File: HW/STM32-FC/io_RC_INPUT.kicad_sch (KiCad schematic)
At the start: 9 parts, among them J6 PWM_Conn_3x14, J7 ZH 1.5mm 3P, J8 ZH 1.5mm 4P, Q2 S9013

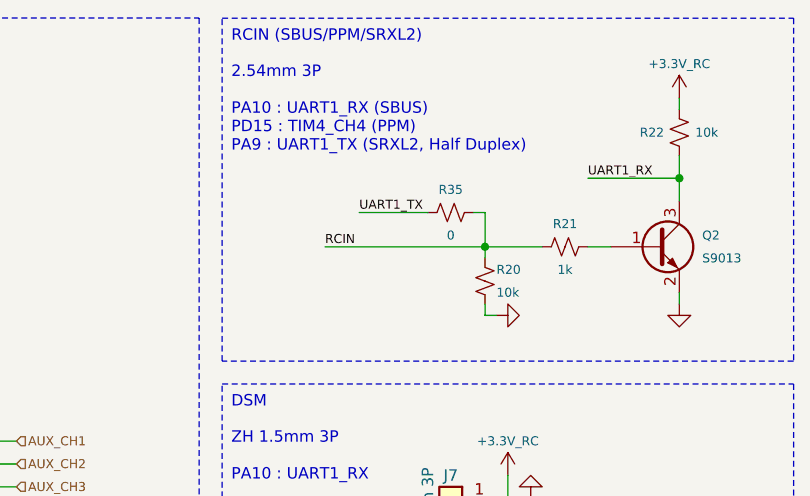
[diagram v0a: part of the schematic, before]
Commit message: 2025.02.05 PCB routing done
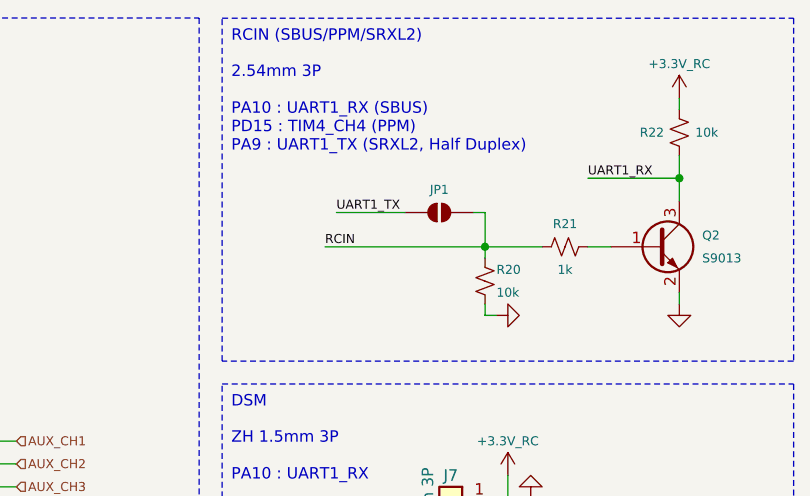
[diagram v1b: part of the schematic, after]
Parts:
- removed R35: 0, Resistor_SMD:R_0402_1005Metric, symbol Device:R_Small_US
- added JP1: SolderJumper_2_Open, Jumper:SolderJumper-2_P1.3mm_Open_TrianglePad1.0x1.5mm, symbol Jumper:SolderJumper_2_Open
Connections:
- net PPM_IN: now also JP1.2 (B)
- net UART1_TX: now also JP1.1 (A)
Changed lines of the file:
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@@
 	(title_block
 		(title "RC_INPUT")
-		(date "2025-01-03")
+		(date "2025-02-05")
 		(rev "A")
 		(company "NARAE")
@@
 	(wire
 		(pts
-			(xy 104.14 34.29) (xy 111.76 34.29)
+			(xy 101.6 34.29) (xy 109.22 34.29)
 		)
 		(stroke
@@
 	)
 	(label "UART1_TX"
-		(at 104.14 34.29 0)
+		(at 101.6 34.29 0)
 		(effects
 			(font
@@
 				(path "/8d4cc317-3933-4aa6-844b-8c5c635e89c7/77caf73d-b7f5-48a6-9de3-ef3df69ee7d9"
 					(reference "#PWR076")
-					(unit 1)
-				)
-			)
-		)
-	)
-	(symbol
-		(lib_id "Device:R_Small_US")
-		(at 114.3 34.29 90)
-		(unit 1)
-		(exclude_from_sim no)
-		(in_bom yes)
-		(on_board yes)
-		(dnp no)
-		(property "Reference" "R35"
-			(at 114.3 31.75 90)
-			(effects
-				(font
-					(size 1 1)
-				)
-			)
-		)
-		(property "Value" "0"
-			(at 114.3 36.83 90)
-			(effects
-				(font
-					(size 1 1)
-				)
-			)
-		)
-		(property "Footprint" "Resistor_SMD:R_0402_1005Metric"
-			(at 114.3 34.29 0)
-			(effects
-				(font
-					(size 1.27 1.27)
-				)
-				(hide yes)
-			)
-		)
-		(property "Datasheet" "~"
-			(at 114.3 34.29 0)
-			(effects
-				(font
-					(size 1.27 1.27)
-				)
-				(hide yes)
-			)
-		)
-		(property "Description" "Resistor, small US symbol"
-			(at 114.3 34.29 0)
-			(effects
-				(font
-					(size 1.27 1.27)
-				)
-				(hide yes)
-			)
-		)
-		(property "Availability" ""
-			(at 114.3 34.29 0)
-			(effects
-				(font
-					(size 1.27 1.27)
-				)
-				(hide yes)
-			)
-		)
-		(property "Check_prices" ""
-			(at 114.3 34.29 0)
-			(effects
-				(font
-					(size 1.27 1.27)
-				)
-				(hide yes)
-			)
-		)
-		(property "Description_1" ""
-			(at 114.3 34.29 0)
-			(effects
-				(font
-					(size 1.27 1.27)
-				)
-				(hide yes)
-			)
-		)
-		(property "MF" ""
-			(at 114.3 34.29 0)
-			(effects
-				(font
-					(size 1.27 1.27)
-				)
-				(hide yes)
-			)
-		)
-		(property "MP" ""
-			(at 114.3 34.29 0)
-			(effects
-				(font
-					(size 1.27 1.27)
-				)
-				(hide yes)
-			)
-		)
-		(property "Package" ""
-			(at 114.3 34.29 0)
-			(effects
-				(font
-					(size 1.27 1.27)
-				)
-				(hide yes)
-			)
-		)
-		(property "Price" ""
-			(at 114.3 34.29 0)
-			(effects
-				(font
-					(size 1.27 1.27)
-				)
-				(hide yes)
-			)
-		)
-		(property "SnapEDA_Link" ""
-			(at 114.3 34.29 0)
-			(effects
-				(font
-					(size 1.27 1.27)
-				)
-				(hide yes)
-			)
-		)
-		(property "Sim.Device" ""
-			(at 114.3 34.29 0)
-			(effects
-				(font
-					(size 1.27 1.27)
-				)
-				(hide yes)
-			)
-		)
-		(property "Sim.Pins" ""
-			(at 114.3 34.29 0)
-			(effects
-				(font
-					(size 1.27 1.27)
-				)
-				(hide yes)
-			)
-		)
-		(pin "1"
-		)
-		(pin "2"
-		)
-		(instances
-			(project "STM32-FC"
-				(path "/8d4cc317-3933-4aa6-844b-8c5c635e89c7/77caf73d-b7f5-48a6-9de3-ef3df69ee7d9"
-					(reference "R35")
 					(unit 1)
 				)
@@
 					(unit 1)
 				)
+			)
+		)
+	)
+	(symbol
+		(lib_id "Jumper:SolderJumper_2_Open")
+		(at 113.03 34.29 0)
+		(unit 1)
+		(exclude_from_sim yes)
+		(in_bom no)
+		(on_board yes)
+		(dnp no)
+		(property "Reference" "JP1"
+			(at 113.03 31.75 0)
+			(effects
+				(font
+					(size 1 1)
+				)
+			)
+		)
+		(property "Value" "SolderJumper_2_Open"
+			(at 113.03 30.48 0)
+			(effects
+				(font
+					(size 1.27 1.27)
+				)
+				(hide yes)
+			)
+		)
+		(property "Footprint" "Jumper:SolderJumper-2_P1.3mm_Open_TrianglePad1.0x1.5mm"
+			(at 113.03 34.29 0)
+			(effects
+				(font
+					(size 1.27 1.27)
+				)
+				(hide yes)
+			)
+		)
+		(property "Datasheet" "~"
+			(at 113.03 34.29 0)
+			(effects
+				(font
+					(size 1.27 1.27)
+				)
+				(hide yes)
+			)
+		)
+		(property "Description" "Solder Jumper, 2-pole, open"
+			(at 113.03 34.29 0)
+			(effects
+				(font
+					(size 1.27 1.27)
+				)
+				(hide yes)
+			)
+		)
+		(pin "2"
+		)
+		(pin "1"
+		)
+		(instances
+			(project ""
+				(path "/8d4cc317-3933-4aa6-844b-8c5c635e89c7/77caf73d-b7f5-48a6-9de3-ef3df69ee7d9"
+					(reference "JP1")
+					(unit 1)
+				)

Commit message: 2025.02.06 PCB routing done v2
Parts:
- J6: LCSC (none) -> C3327492
- J7: LCSC (none) -> C72591
- J8: LCSC (none) -> C485354
- JP1: LCSC (none) -> C161692
- Q2: LCSC (none) -> C111269
- R19, R20, R22: LCSC (none) -> C25531
- R21: LCSC (none) -> C11702
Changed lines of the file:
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@@
+			)
+		)
+		(property "LCSC" "C25531"
+			(at 54.61 104.14 0)
+			(effects
+				(font
+					(size 1.27 1.27)
+				)
+				(hide yes)
 			)
 		)
@@
 		)
 		(property "Sim.Pins" ""
+			(at 118.11 41.91 0)
+			(effects
+				(font
+					(size 1.27 1.27)
+				)
+				(hide yes)
+			)
+		)
+		(property "LCSC" "C25531"
 			(at 118.11 41.91 0)
 			(effects
@@
 			)
 		)
+		(property "LCSC" "C111269"
+			(at 137.16 38.1 0)
+			(effects
+				(font
+					(size 1.27 1.27)
+				)
+				(hide yes)
+			)
+		)
 		(pin "1"
 		)
@@
 		)
 		(property "Sim.Pins" ""
+			(at 115.57 101.6 0)
+			(effects
+				(font
+					(size 1.27 1.27)
+				)
+				(hide yes)
+			)
+		)
+		(property "LCSC" "C485354"
 			(at 115.57 101.6 0)
 			(effects
@@
 			)
 		)
+		(property "LCSC" "C25531"
+			(at 139.7 25.4 0)
+			(effects
+				(font
+					(size 1.27 1.27)
+				)
+				(hide yes)
+			)
+		)
 		(pin "1"
 		)
@@
 			)
 		)
+		(property "LCSC" "C72591"
+			(at 114.3 68.58 0)
+			(effects
+				(font
+					(size 1.27 1.27)
+				)
+				(hide yes)
+			)
+		)
 		(pin "1"
 		)
@@
 			)
 		)
+		(property "LCSC" "C11702"
+			(at 127 38.1 0)
+			(effects
+				(font
+					(size 1.27 1.27)
+				)
+				(hide yes)
+			)
+		)
 		(pin "1"
 		)
@@
 		)
 		(property "Description" "Solder Jumper, 2-pole, open"
+			(at 113.03 34.29 0)
+			(effects
+				(font
+					(size 1.27 1.27)
+				)
+				(hide yes)
+			)
+		)
+		(property "LCSC" "C161692"
 			(at 113.03 34.29 0)
 			(effects
@@
 			(at 54.61 63.5 0)
 			(effects
+				(font
+					(size 1.27 1.27)
+				)
+				(hide yes)
+			)
+		)
+		(property "LCSC" "C3327492"
+			(at 54.61 63.5 0)
+			(effects
